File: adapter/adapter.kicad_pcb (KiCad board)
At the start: 2 copper layers, 96 x 46 mm, 18 parts, among them J1 Conn_02x13_Top_Bottom, J10 Screw_Terminal_01x02, J11 Screw_Terminal_01x02, J12 Screw_Terminal_01x02, J13 Screw_Terminal_01x02, J14 Screw_Terminal_01x02, J2 Screw_Terminal_01x02, J3 Screw_Terminal_01x02, J4 Screw_Terminal_01x02, J5 Screw_Terminal_01x02, J6 Screw_Terminal_01x02, J7 Screw_Terminal_01x02, J8 Screw_Terminal_01x02, J9 Screw_Terminal_01x02

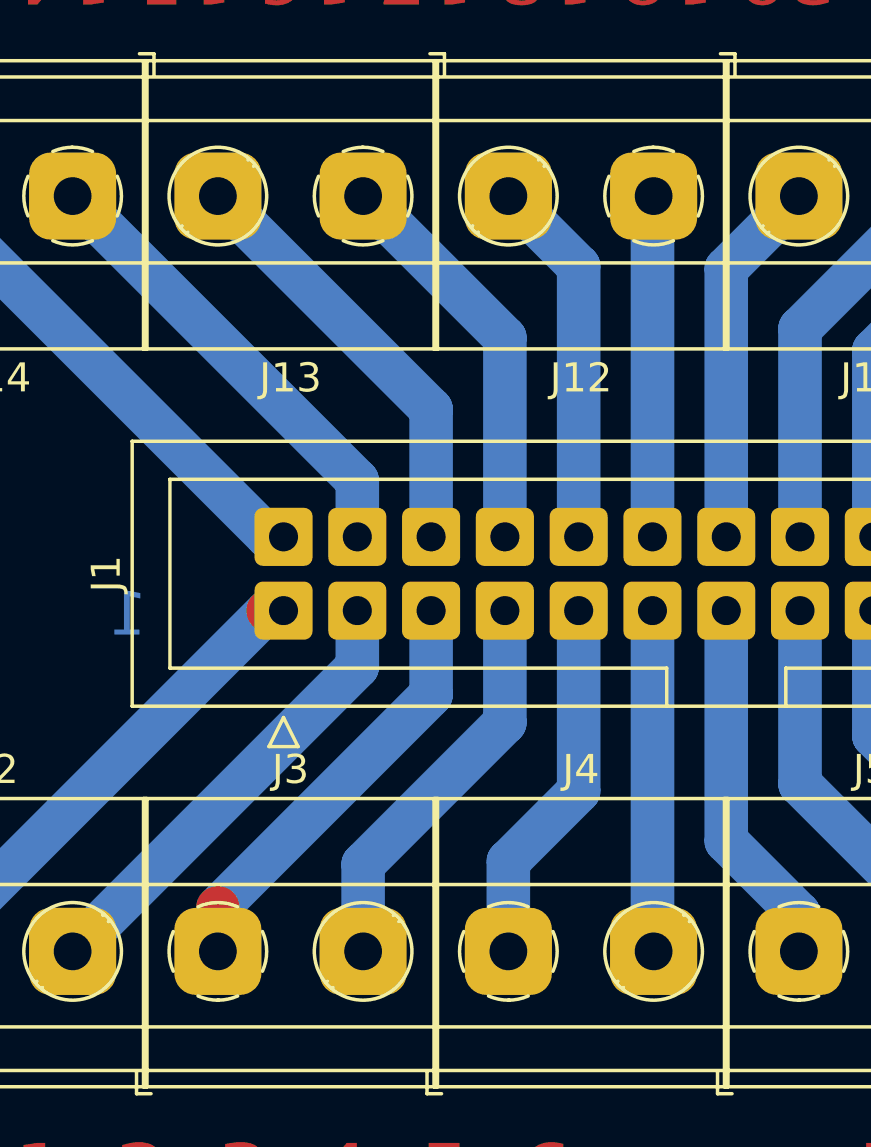
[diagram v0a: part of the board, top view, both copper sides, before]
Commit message: Fix small mistakes
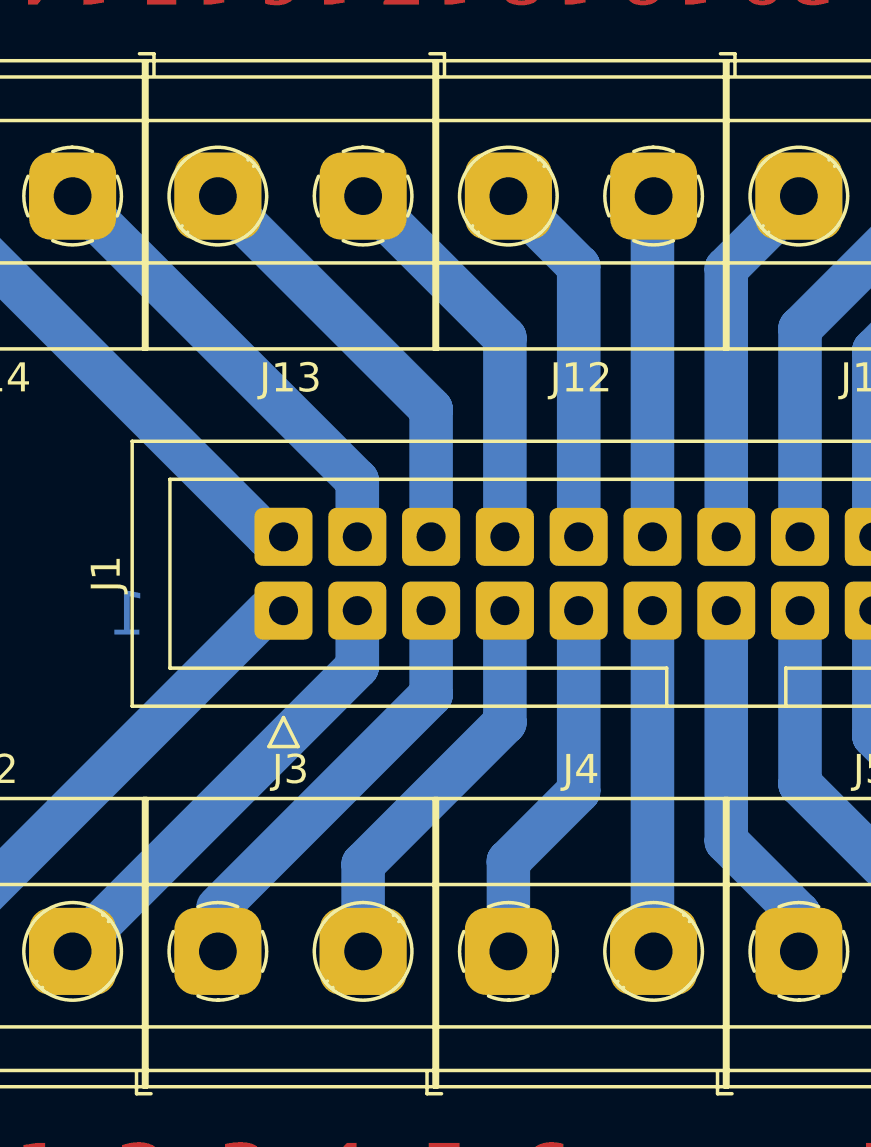
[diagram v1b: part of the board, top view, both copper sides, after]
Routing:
- net /3: track 14.8 -> 13.3 mm
- net /1: track 17.1 -> 16.6 mm

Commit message: Checked if it still works in KiCAD 8 and updated
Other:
- net class Default removed
